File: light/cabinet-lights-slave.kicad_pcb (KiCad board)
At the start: 2 copper layers, 50 x 50 mm, 13 parts, among them J1 NORTH, J2 EAST, J3 SOUTH, J4 WEST, Q1 BC817-40

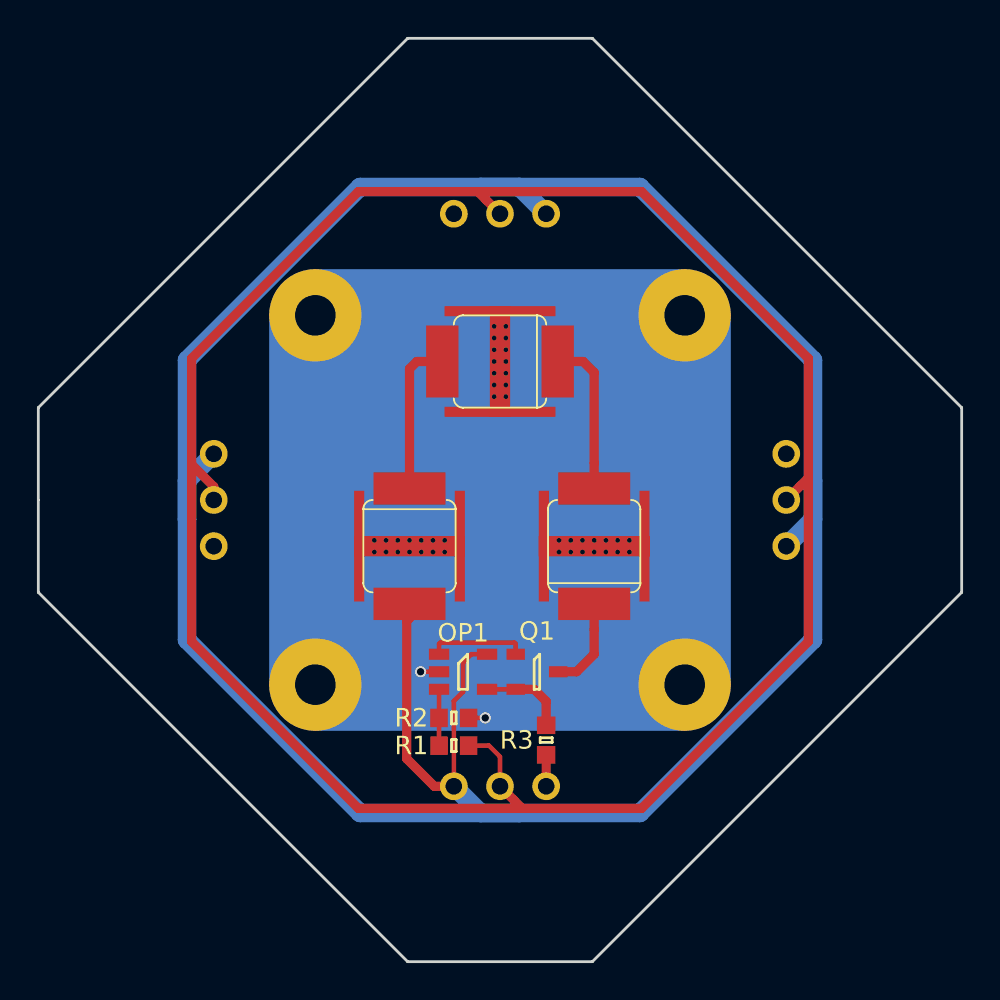
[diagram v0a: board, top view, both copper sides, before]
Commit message: Mounting holes, some track shenanigans
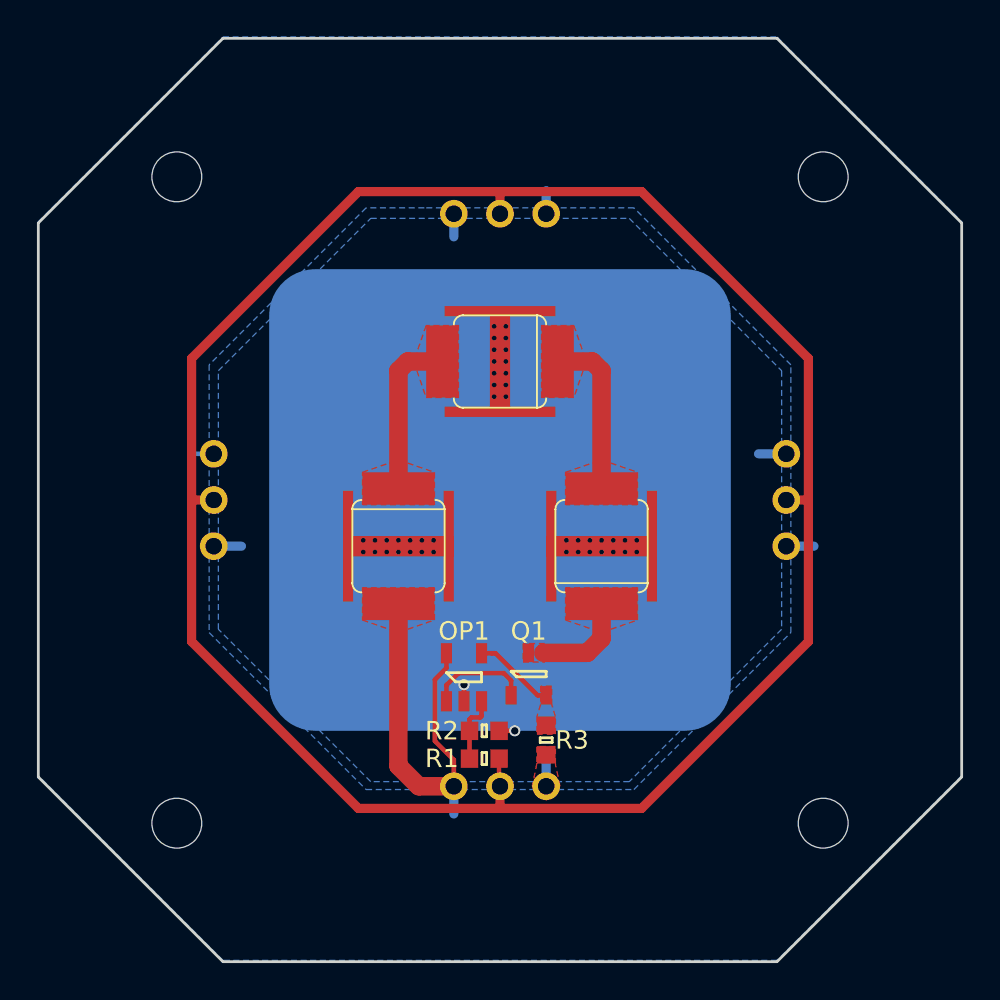
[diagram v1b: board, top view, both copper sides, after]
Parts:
- added X1: MOUNT, Mounting_Holes:MountingHole_2.7mm_M2.5, F.Cu at (37.5, 72.5)
- added X2: MOUNT, Mounting_Holes:MountingHole_2.7mm_M2.5, F.Cu at (37.5, 37.5)
- added X3: MOUNT, Mounting_Holes:MountingHole_2.7mm_M2.5, F.Cu at (72.5, 72.5)
- added X4: MOUNT, Mounting_Holes:MountingHole_2.7mm_M2.5, F.Cu at (72.5, 37.5)
- moved R1 1.79 mm to (54.1, 69.0)
- moved R2 1.79 mm to (54.1, 67.5)
- moved D1 0.60 mm to (49.5, 57.5)
- moved Q1 0.47 mm to (56.5, 64.4), turned to 90 degrees
- moved D3 0.40 mm to (60.5, 57.5)
- moved OP1 0.30 mm to (53.0, 64.6), turned to 90 degrees
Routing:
- net +12V: track 150.2 -> 25.6 mm
- net /DIM: track 123.5 -> 118.8 mm
- net GND: track 3.90 -> 7.80 mm
- net /DIM/100: track 3.05 -> 3.65 mm
- net Net-(D1-Pad1): track 8.42 -> 8.96 mm
- added copper zone on B.Cu, net +12V
- added copper zone on F.Cu, net +12V
- added copper zone on F.Cu, net /SENSE
- added copper zone on F.Cu, net GND
- added copper zone on F.Cu, net Net-(D1-Pad1)
- added copper zone on F.Cu, net Net-(D2-Pad1)
- added copper zone on F.Cu, net Net-(D3-Pad1)
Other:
- outline, holes or cut-outs redrawn
